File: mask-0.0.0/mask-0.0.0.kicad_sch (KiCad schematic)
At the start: 18 parts, among them J3 Conn_ARM_JTAG_SWD_10, Q1 IRLML2502, U1 NORA-B10x, U2 MCP1703A-3302_SOT23

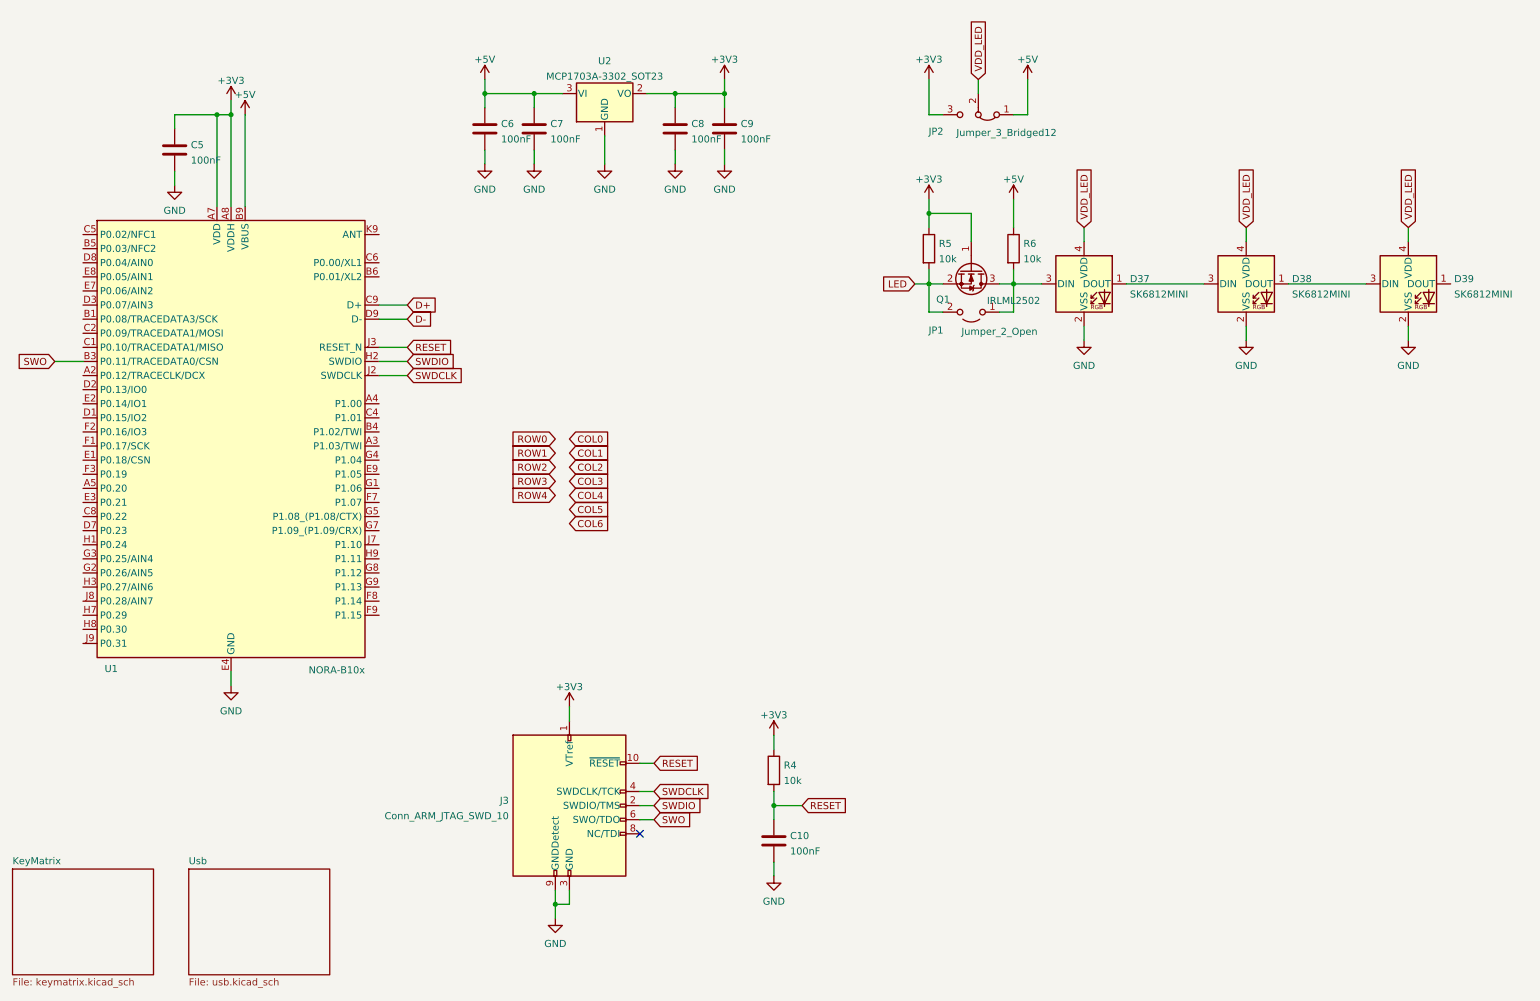
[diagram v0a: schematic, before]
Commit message: udpate routing
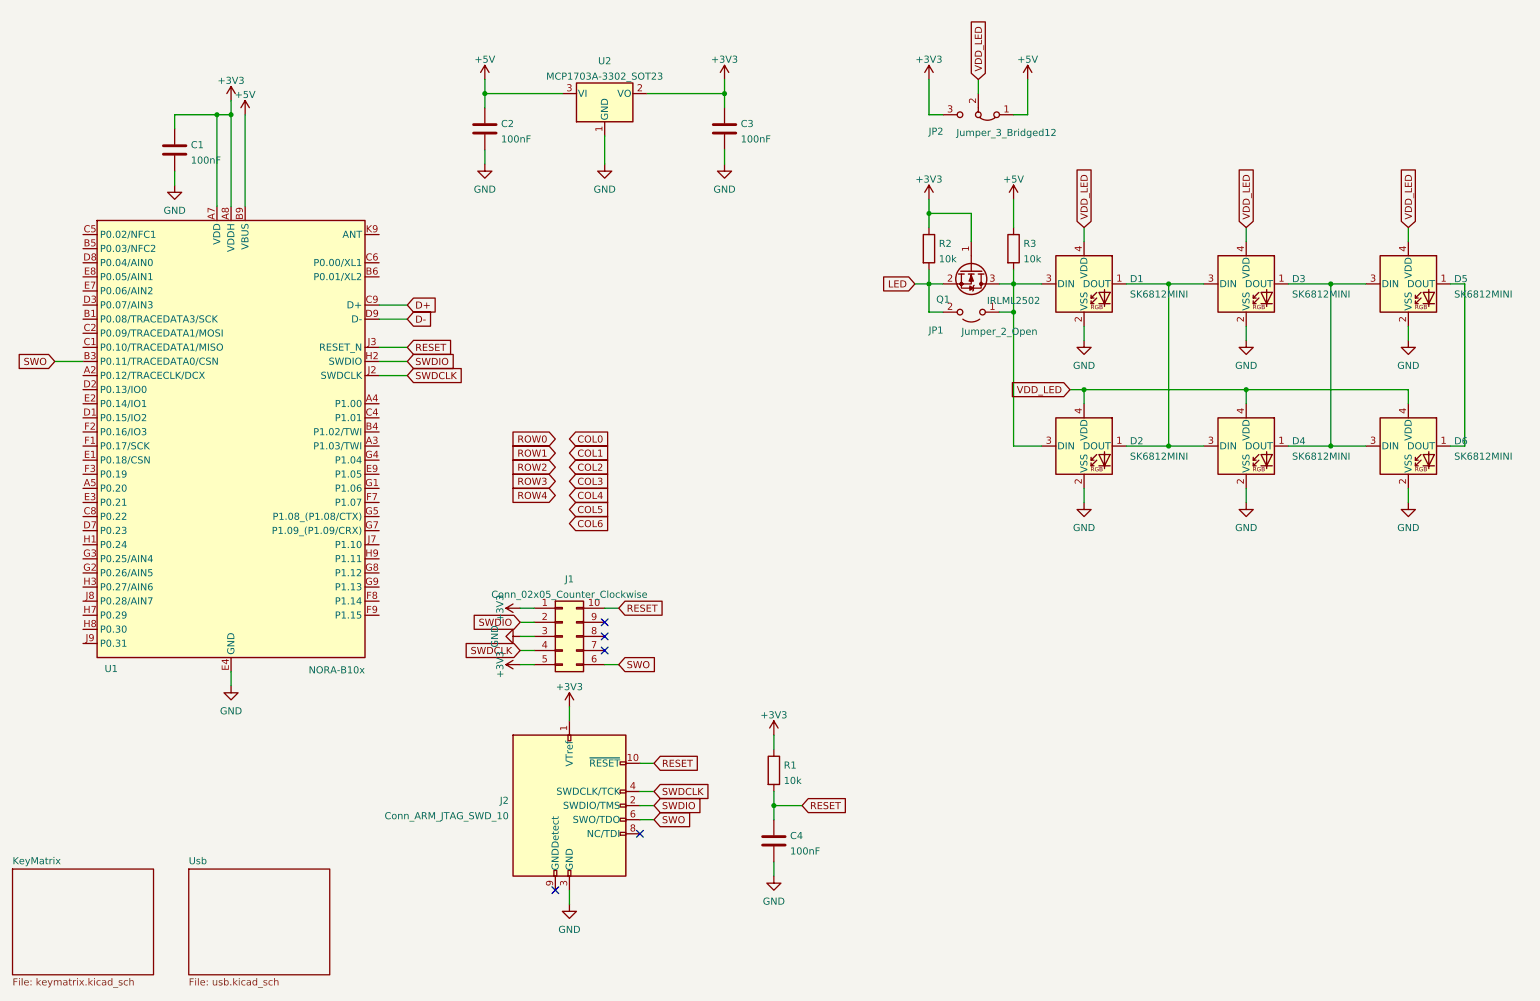
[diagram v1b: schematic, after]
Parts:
- removed C7, C8: 100nF, Capacitor_SMD:C_0603_1608Metric, symbol Device:C
- added D2, D4, D6: SK6812MINI, LED_SMD:LED_SK6812MINI_PLCC4_3.5x3.5mm_P1.75mm, symbol LED:SK6812MINI
- added J1: Conn_02x05_Counter_Clockwise, Connector:Tag-Connect_TC2050-IDC-NL_2x05_P1.27mm_Vertical, symbol Connector_Generic:Conn_02x05_Counter_Clockwise
- renumbered C5 to C1, C6 to C2, C9 to C3, C10 to C4, D37 to D1, D38 to D3, D39 to D5, J3 to J2, R4 to R1, R5 to R2, R6 to R3
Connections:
- net +3V3: now also J1.1 (Pin_1), J1.5 (Pin_5)
- net GND: now also D2.2 (VSS), D4.2 (VSS), D6.2 (VSS), J1.3 (Pin_3); no longer J2.9 (GNDDetect)
- net RESET: now also J1.10 (Pin_10)
- net SWDCLK: now also J1.4 (Pin_4)
- net SWDIO: now also J1.2 (Pin_2)
- net SWO: now also J1.6 (Pin_6)
- net VDD_LED: now also D2.4 (VDD), D4.4 (VDD), D6.4 (VDD)
- net at D3.1 (DOUT), D5.3 (DIN): now also D4.1 (DOUT), D6.3 (DIN)
- net at D1.1 (DOUT), D3.3 (DIN): now also D2.1 (DOUT), D4.3 (DIN)
- net at D1.3 (DIN), JP1.1 (A), Q1.3 (D)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: now also D2.3 (DIN)
- net at D5.1 (DOUT): now also D6.1 (DOUT)
- no-connect marks 1 -> 5
